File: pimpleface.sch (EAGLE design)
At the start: 31 parts, among them J1 B06B-HCMKK, J2 POWERPOLE_POWER45A_DRILL, J3 POWERPOLE_POWER45A_DRILL

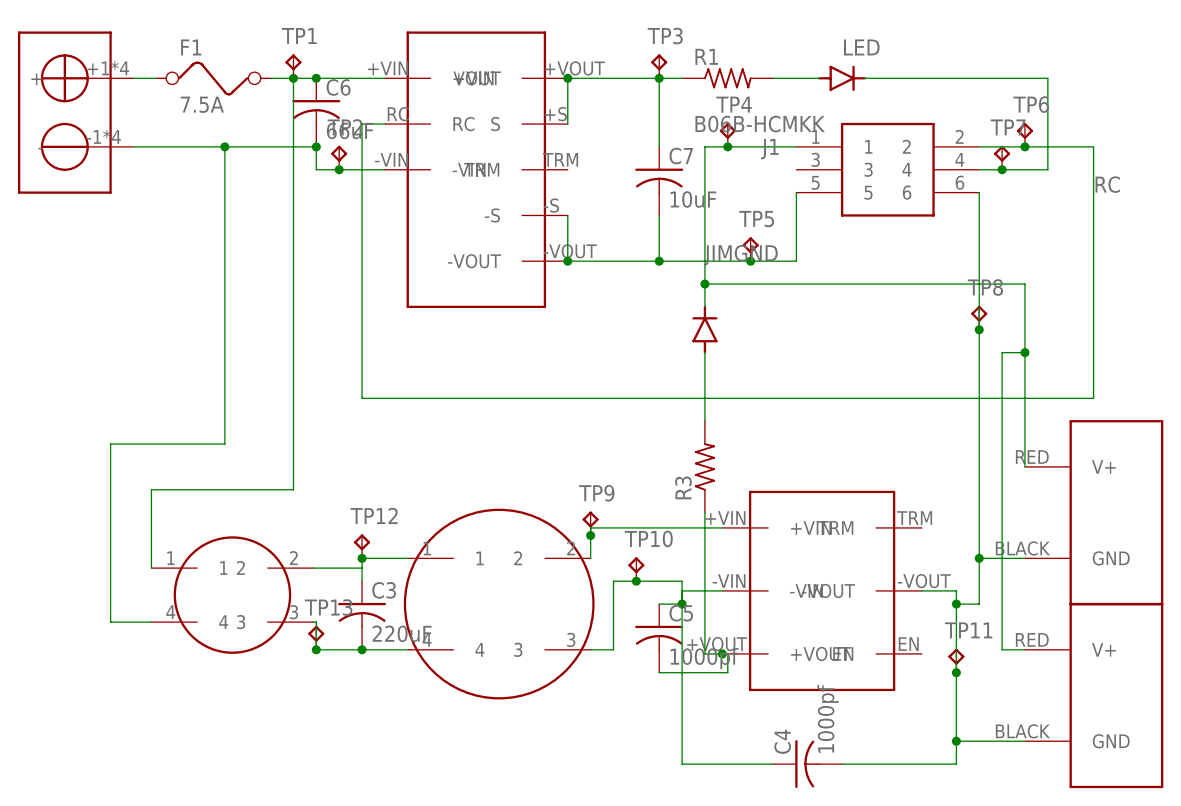
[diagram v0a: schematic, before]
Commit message: Add files via upload
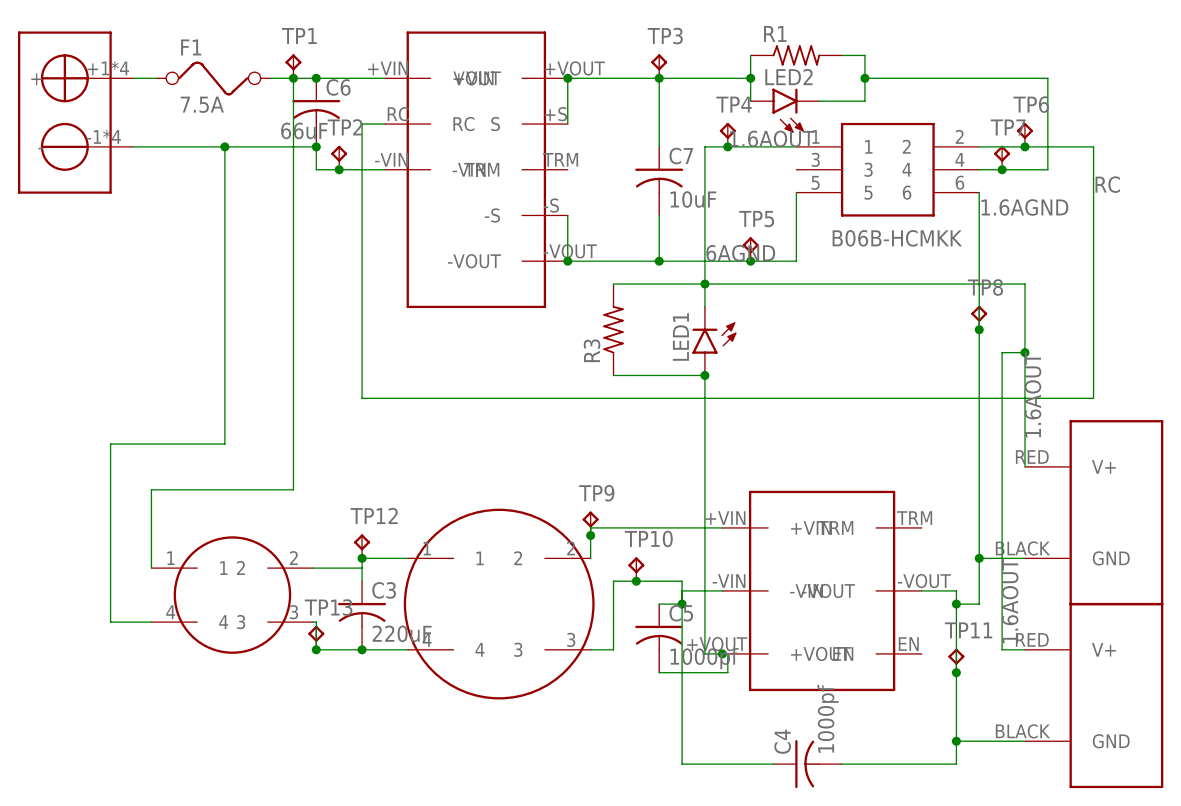
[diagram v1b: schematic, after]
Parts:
- removed D1, D3: BYV95, diode:BYV95
- added LED1, LED2: (no value), led:LEDCHIP-LED0603
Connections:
- net JIMGND renamed 6AGND
- net N$8 renamed 1.6AGND
- removed net N$22: D3.C, J1.1, J2.V+, J3.V+, TP4.TP
- removed net N$34: D3.A, R3.2
- removed net N$4: D1.A, R1.2
- new net 1.6AOUT: J1.1, J2.V+, J3.V+, LED1.C, R3.2, TP4.TP
- net LED: now also LED2.C, R1.2; no longer D1.C
- net N$1: now also LED2.A
- net N$9: now also LED1.A
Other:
- moved on the sheet: R1, R3
